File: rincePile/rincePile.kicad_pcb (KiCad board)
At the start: 2 copper layers, 19.7 x 19.7 mm, 9 parts, among them J1 Conn_01x02_Male, J2 Conn_01x02_Male, J3 Conn_01x04_Male, Q1 BC547

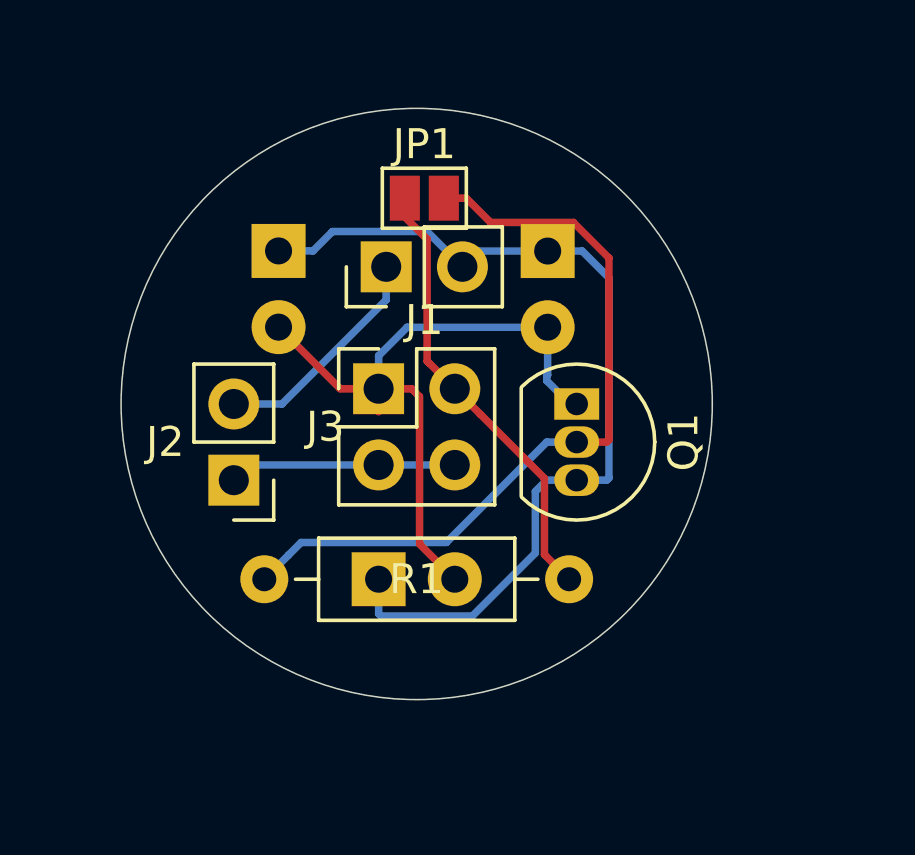
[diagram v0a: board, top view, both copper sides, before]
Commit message: update PCB creation des gerber et fichiers de percage
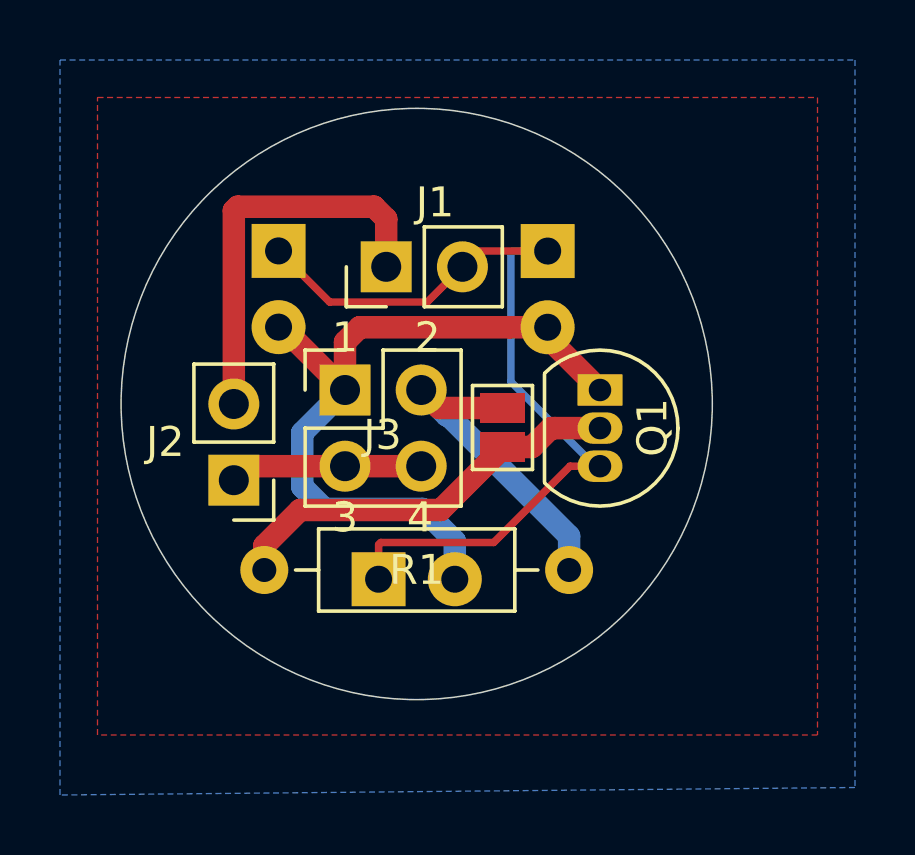
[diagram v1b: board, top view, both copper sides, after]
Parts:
- moved JP1 8.07 mm to (107.0, -17.2), turned to 270 degrees
- moved J3 1.12 mm to (101.8, -18.5)
- moved Q1 0.91 mm to (110.2, -18.5)
- moved R1 0.31 mm to (99.1, -12.5)
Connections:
- net Net-(D1-Pad1) renamed GND
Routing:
- net Net-(JP1-Pad2): track 26.0 -> 13.6 mm
- net Net-(J1-Pad1): track 7.62 -> 13.3 mm
- net Net-(J3-Pad2): track 16.4 -> 11.0 mm
- net GND: track 31.4 -> 29.7 mm
- net Net-(J2-Pad1): track 7.94 -> 6.44 mm
- net Net-(D1-Pad2): track 24.1 -> 25.4 mm
- added copper zone on B.Cu, net GND
- added copper zone on F.Cu, net GND
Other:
- board text added: "1"
- board text added: "2"
- board text added: "3"
- board text added: "4"
